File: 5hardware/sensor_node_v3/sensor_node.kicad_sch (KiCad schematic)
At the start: 28 parts, among them J1 Conn_01x03, J3 Conn_01x29, SW2 SW_DIP_x04, SW3 SW_Push, SW4 SW_DIP_x04, SW5 RotaryEncoder, SW6 SW_Push, U1 MCP1700x-330xxTO, U7 CH32V003F4P6, U8 ESP32-WROOM-32D

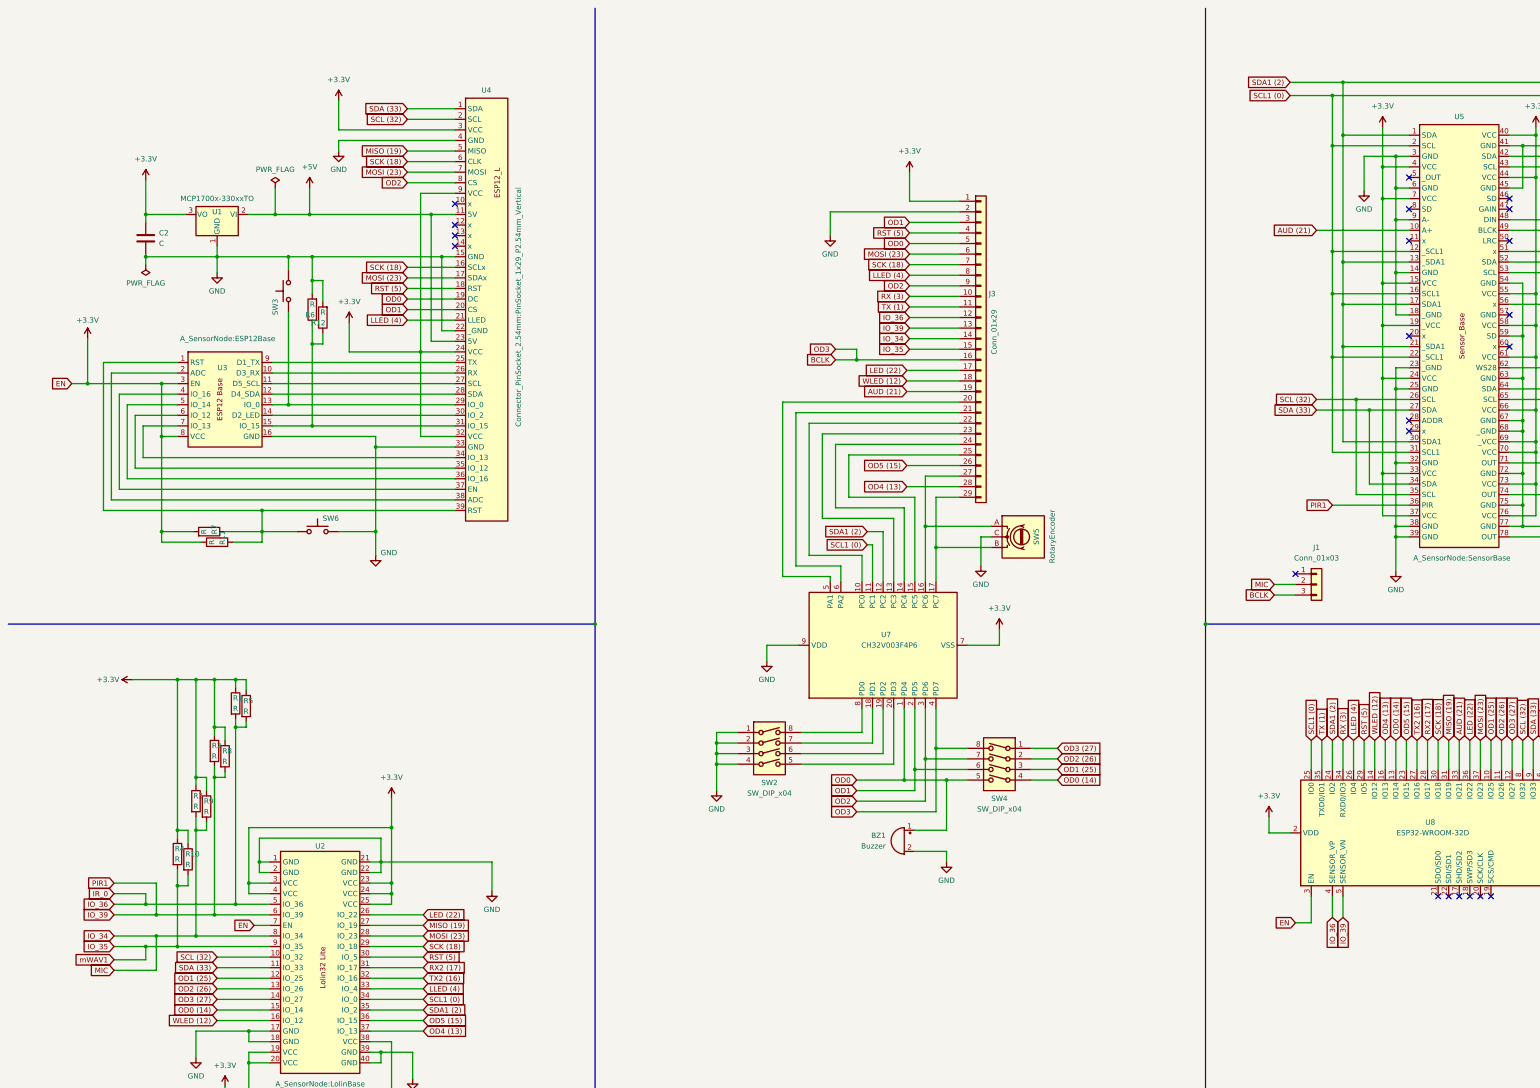
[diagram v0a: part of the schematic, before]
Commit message: update pcb.
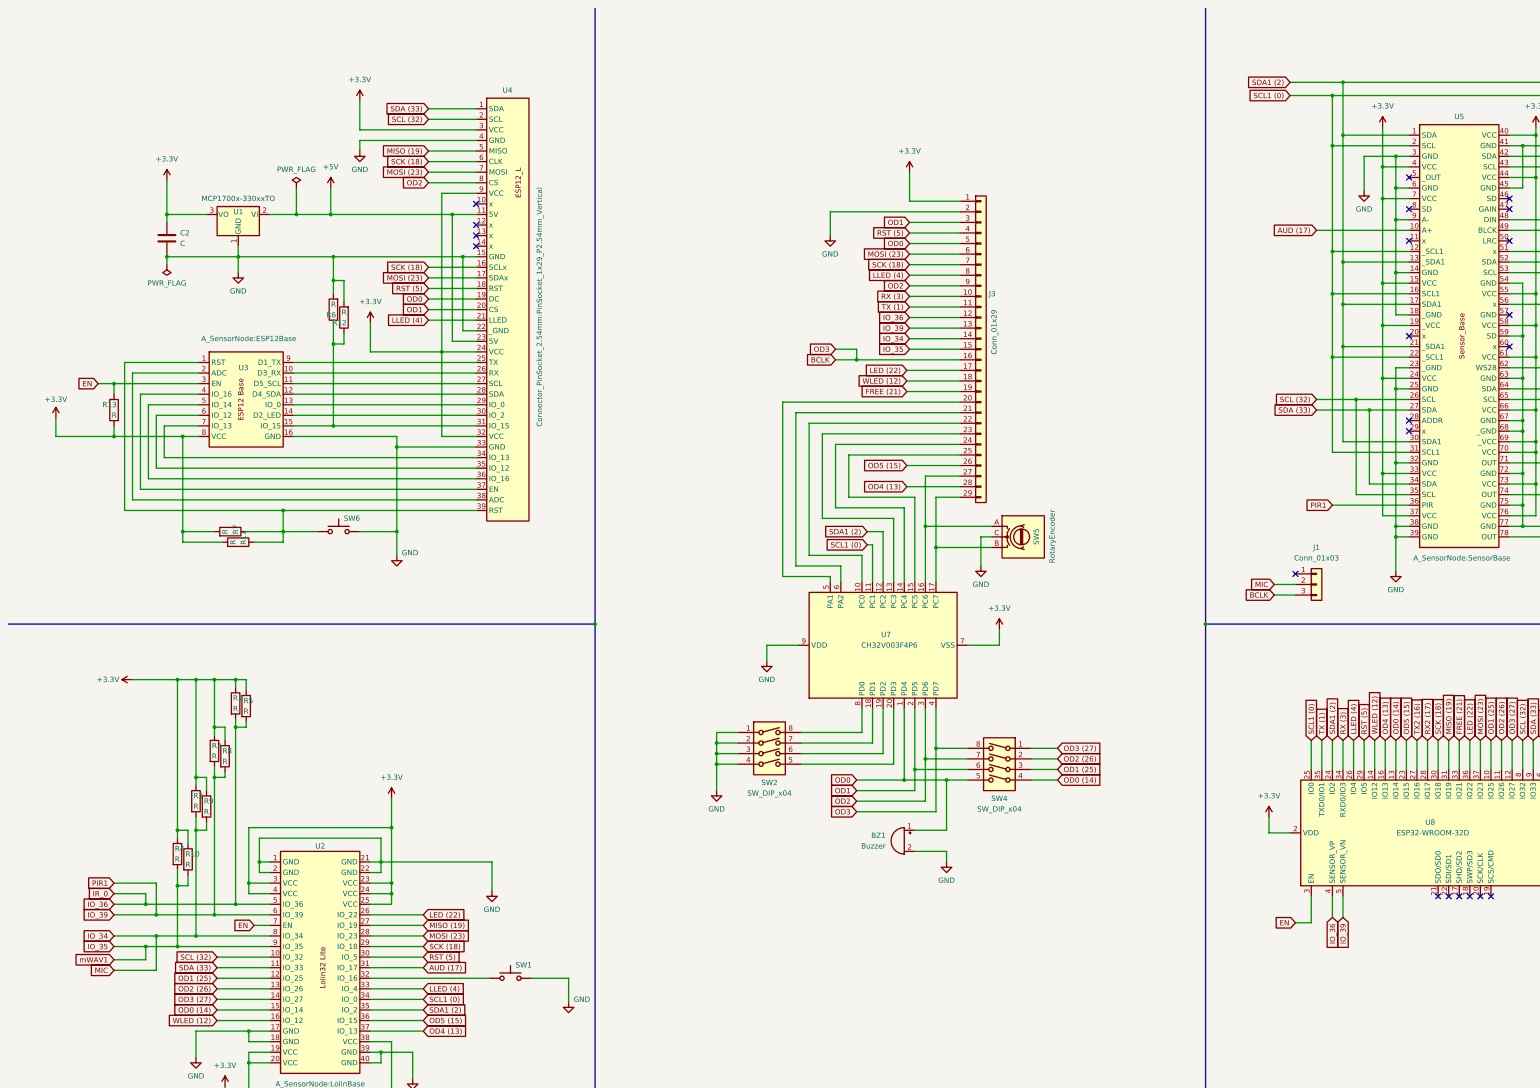
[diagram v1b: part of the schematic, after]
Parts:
- removed SW3: SW_Push, Button_Switch_THT:SW_PUSH_6mm_H7.3mm, symbol Switch:SW_Push
- added R13: R, Connector_PinSocket_2.54mm:PinSocket_1x02_P2.54mm_Vertical, symbol Device:R
- added SW1: SW_Push, Button_Switch_THT:SW_PUSH-12mm, symbol Switch:SW_Push
- SW6: footprint Button_Switch_THT:SW_PUSH-12mm -> Button_Switch_THT:SW_PUSH_6mm_H7.3mm
- U8: footprint RF_Module:ESP32-WROOM-32D -> A_SensorNode:ESP32-WROOM-32D2
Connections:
- net +3.3V: now also R13.2; no longer U2.7 (EN), U3.3 (EN), U8.3 (EN)
- net GND: now also SW1.1
- net RX2 (17): no longer U2.31 (IO_17)
- net TX2 (16): no longer U2.32 (IO_16)
- net AUD (21) renamed FREE (21)
- net FREE (21): no longer U5.10 (A+)
- new net: SW1.2, U2.32 (IO_16)
- new net AUD (17): U2.31 (IO_17), U5.10 (A+)
- new net EN: R13.1, U2.7 (EN), U3.3 (EN), U8.3 (EN)
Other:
- moved on the sheet: C2, R11, R12, R6, R7, SW6, U1, U3, U4

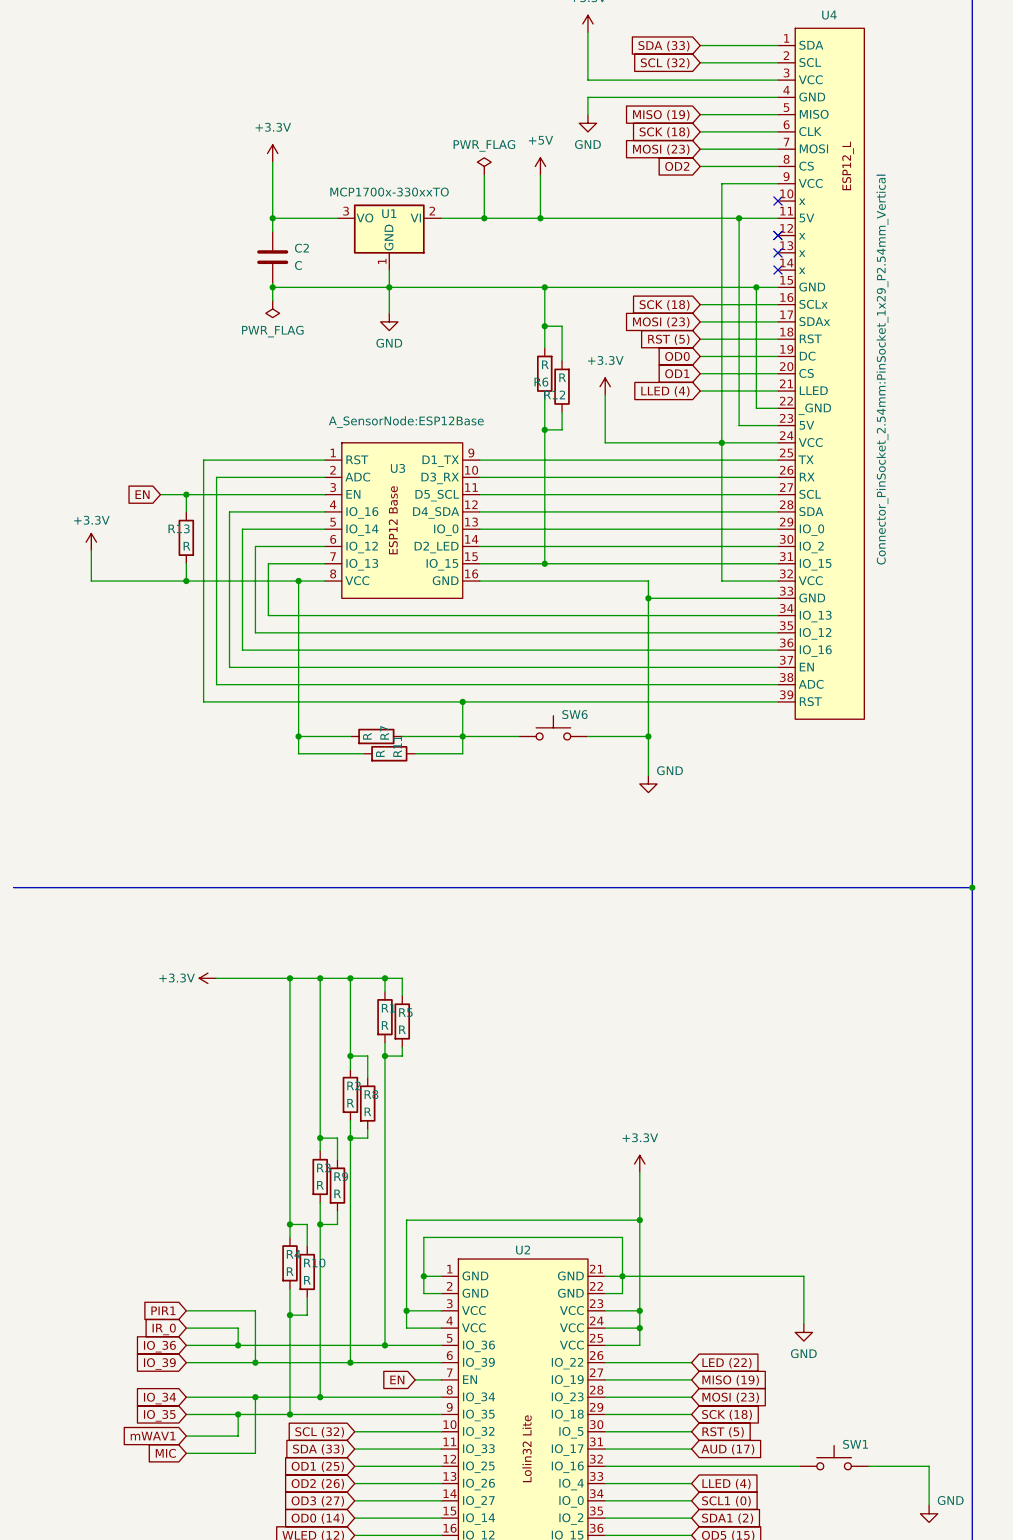
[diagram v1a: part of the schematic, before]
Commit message: update pcb design.
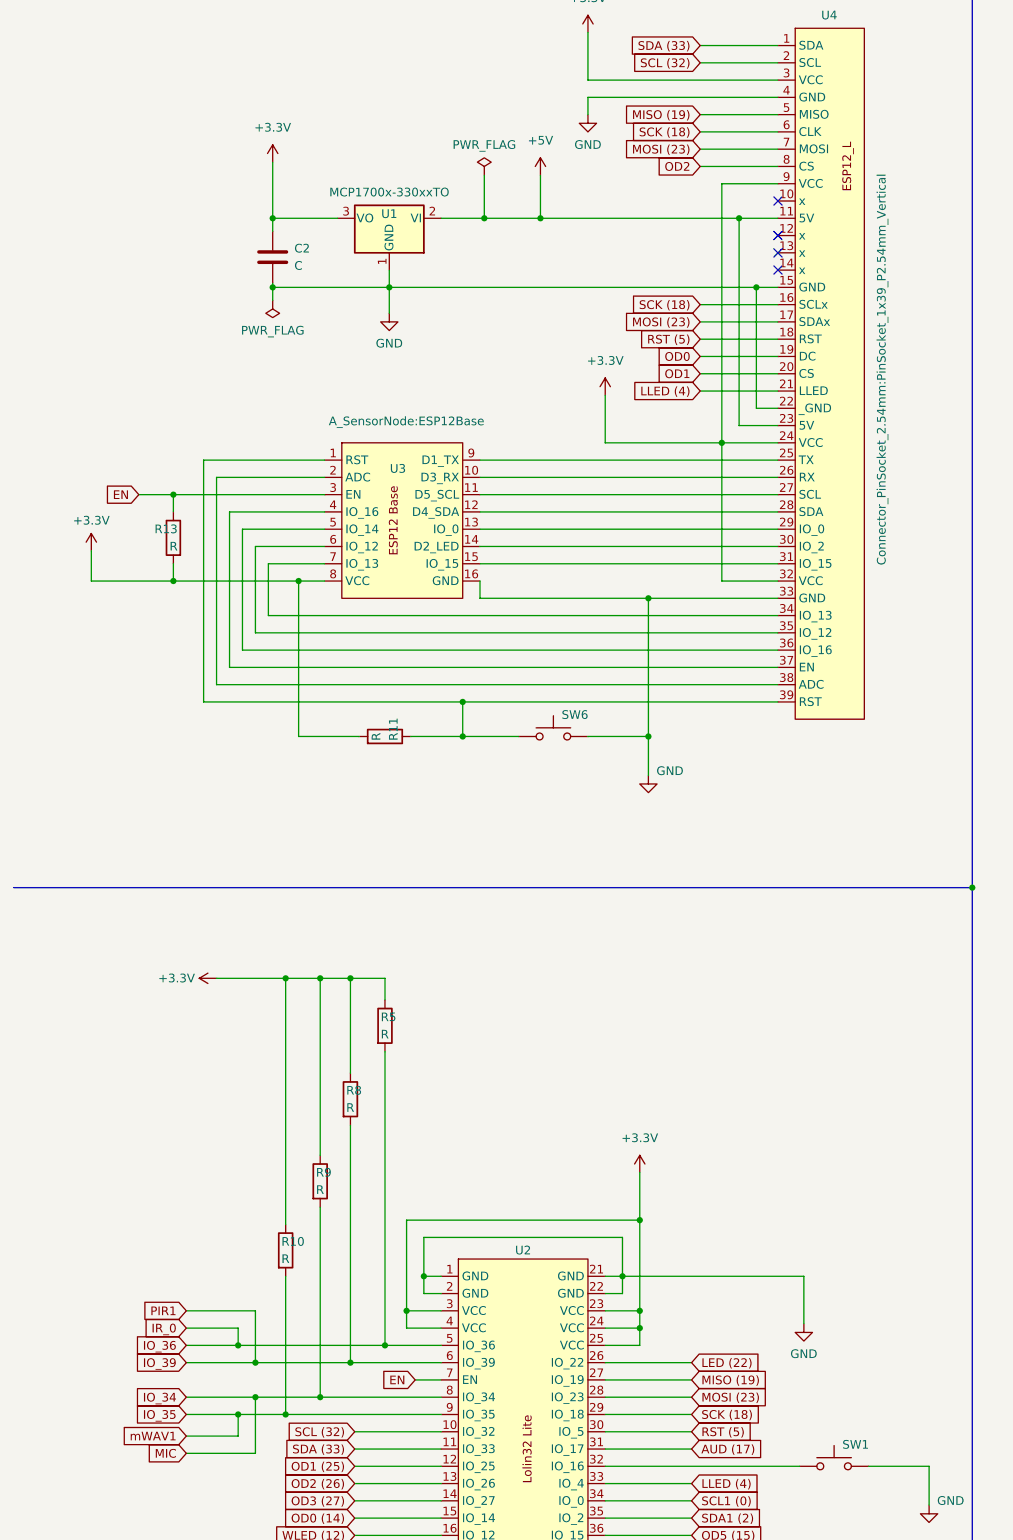
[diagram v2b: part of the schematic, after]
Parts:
- removed R1, R2, R3, R4, R6, R7: R, Connector_PinSocket_2.54mm:PinSocket_1x02_P2.54mm_Vertical, symbol Device:R
- removed R12: R, Resistor_SMD:R_2512_6332Metric, symbol Device:R
- R13: footprint Connector_PinSocket_2.54mm:PinSocket_1x02_P2.54mm_Vertical -> Resistor_SMD:R_2512_6332Metric
- U4: footprint Connector_PinSocket_2.54mm:PinSocket_1x29_P2.54mm_Vertical -> Connector_PinSocket_2.54mm:PinSocket_1x39_P2.54mm_Vertical
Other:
- moved on the sheet: R10, R11, R13, R5, R8, R9
